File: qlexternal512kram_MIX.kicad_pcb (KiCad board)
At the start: 2 copper layers, 97.8 x 40.9 mm, 17 parts, among them J1 QL_SLOT_DIN41612_CARD, J2 QL_SLOT_DIN41612_CARD, SW1 SW_DIP_x02, SW2 SW_SPDT, U1 HM628512BLFP-7, U2 GAL16V8B-25QP, U3 LM1117-5.0

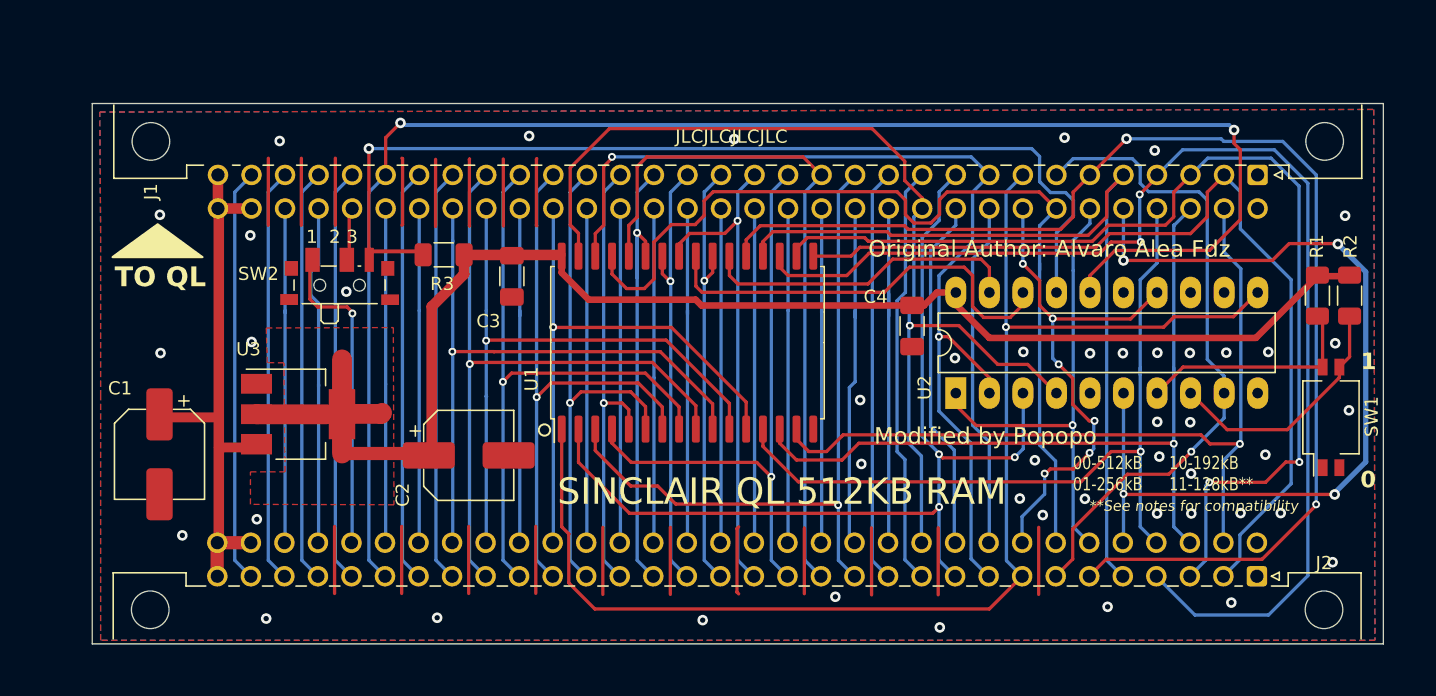
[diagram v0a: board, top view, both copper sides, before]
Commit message: WiP: ultimos cambios locales antes de merge
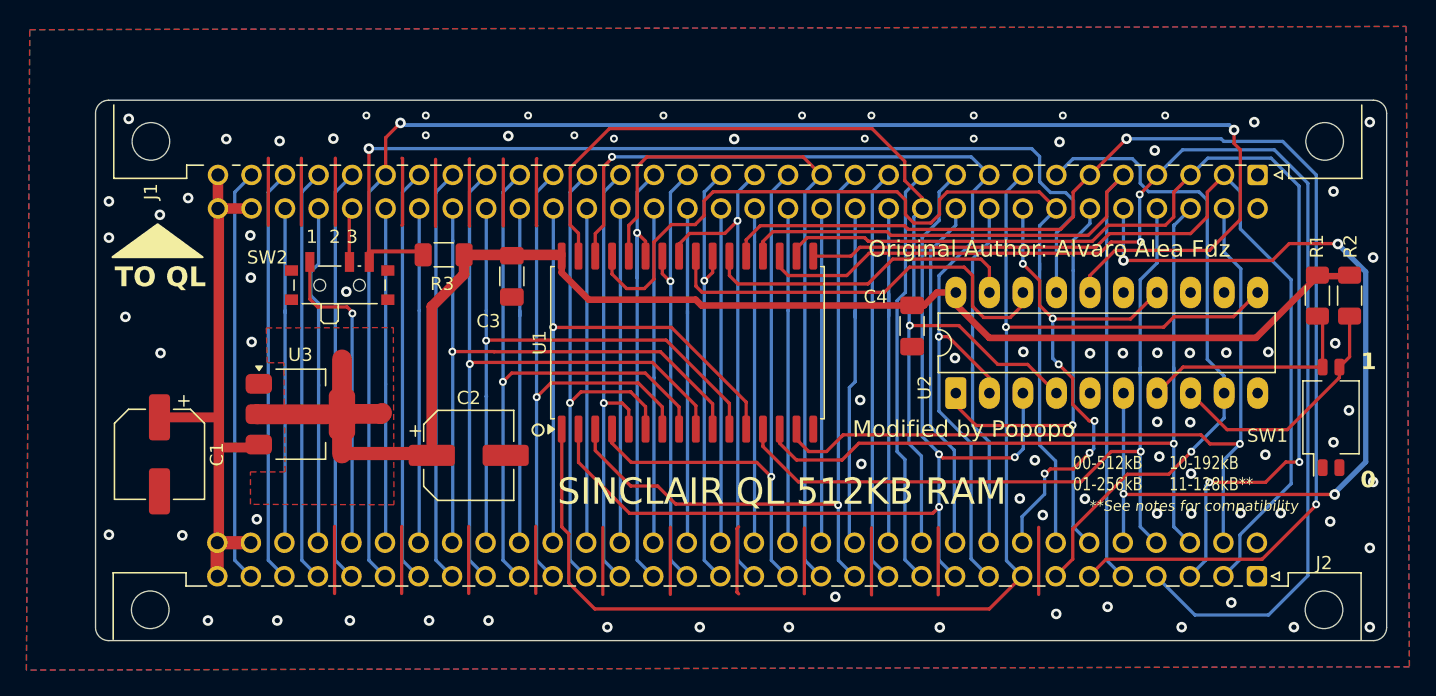
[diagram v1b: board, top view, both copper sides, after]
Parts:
- added QR*****: QR_RAM_CODE, Library:QR_RAM_CODE, B.Cu at (101.8, 75.0)
- C1, C2: footprint Library:CP_Elec_6.3x5.4_Long_Pad -> Capacitor_SMD:CP_Elec_6.3x5.4
- J2: footprint Library:DIN41612_B_2x32_Male_Horizontal_THT -> Connector_DIN:DIN41612_B_2x32_Male_Horizontal_THT
- SW2: footprint Library:SW_SPDT_PCM12 -> Button_Switch_SMD:SW_SPDT_PCM12
- U1: footprint Package_SO:SSOP-32_11.305x20.495mm_P1.27mm -> Package_SO:SOP-32_11.305x20.495mm_P1.27mm
- U3: footprint Library:SOT-223-3_TabPin2_Long_Pads -> Package_TO_SOT_SMD:SOT-223-3_TabPin2
- moved REF** 75.4 mm to (176.2, 79.6)
- moved REF** 63.7 mm to (165.1, 80.6)
- moved REF** 0.75 mm to (116.3, 77.7)
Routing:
- net GND: vias 46 -> 84
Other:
- outline, holes or cut-outs redrawn
- board text added: "REV.1.1"
- board text removed: "JLCJLCJLCJLC"
- board text removed: "REV.1"
